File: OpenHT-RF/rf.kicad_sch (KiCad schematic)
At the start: 22 parts, among them J6 Conn_Coaxial, J7 Conn_01x02, J8 Conn_01x02, X1 ECS-TXO-20CSMV

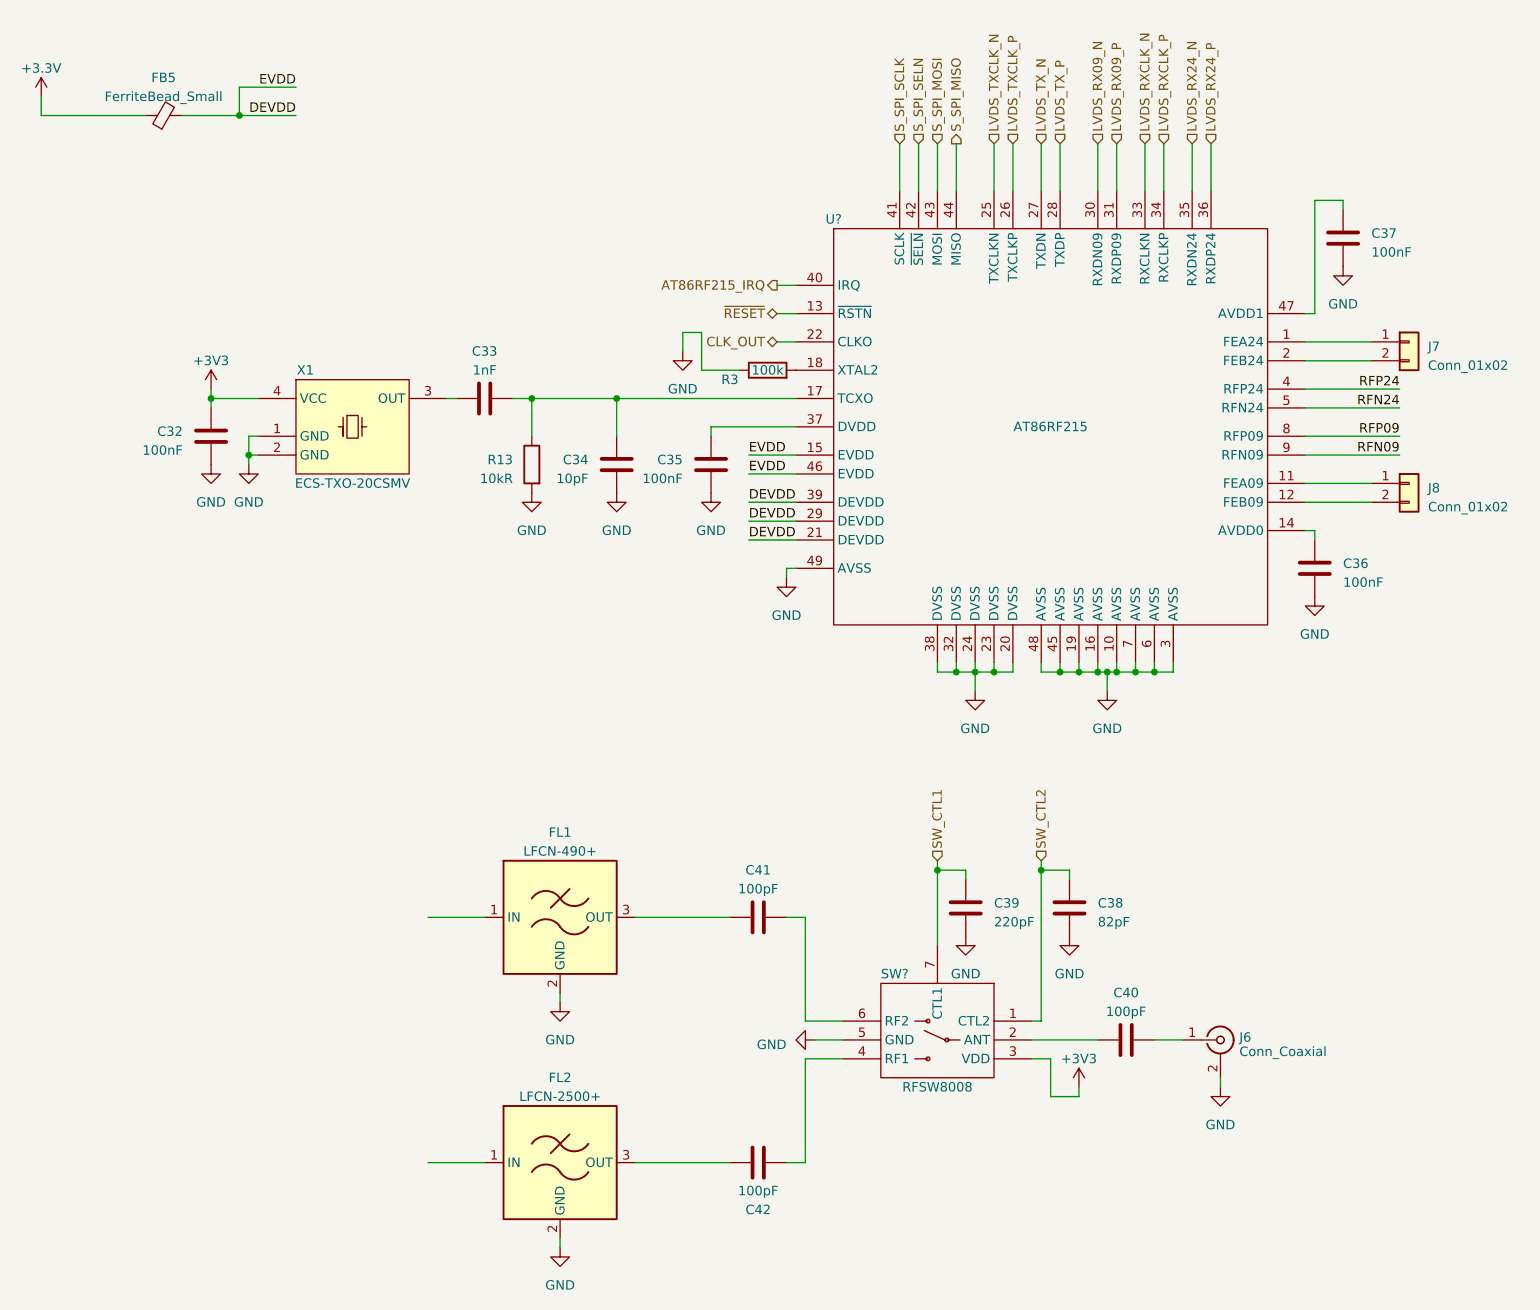
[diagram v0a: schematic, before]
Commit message: Added RF baluns
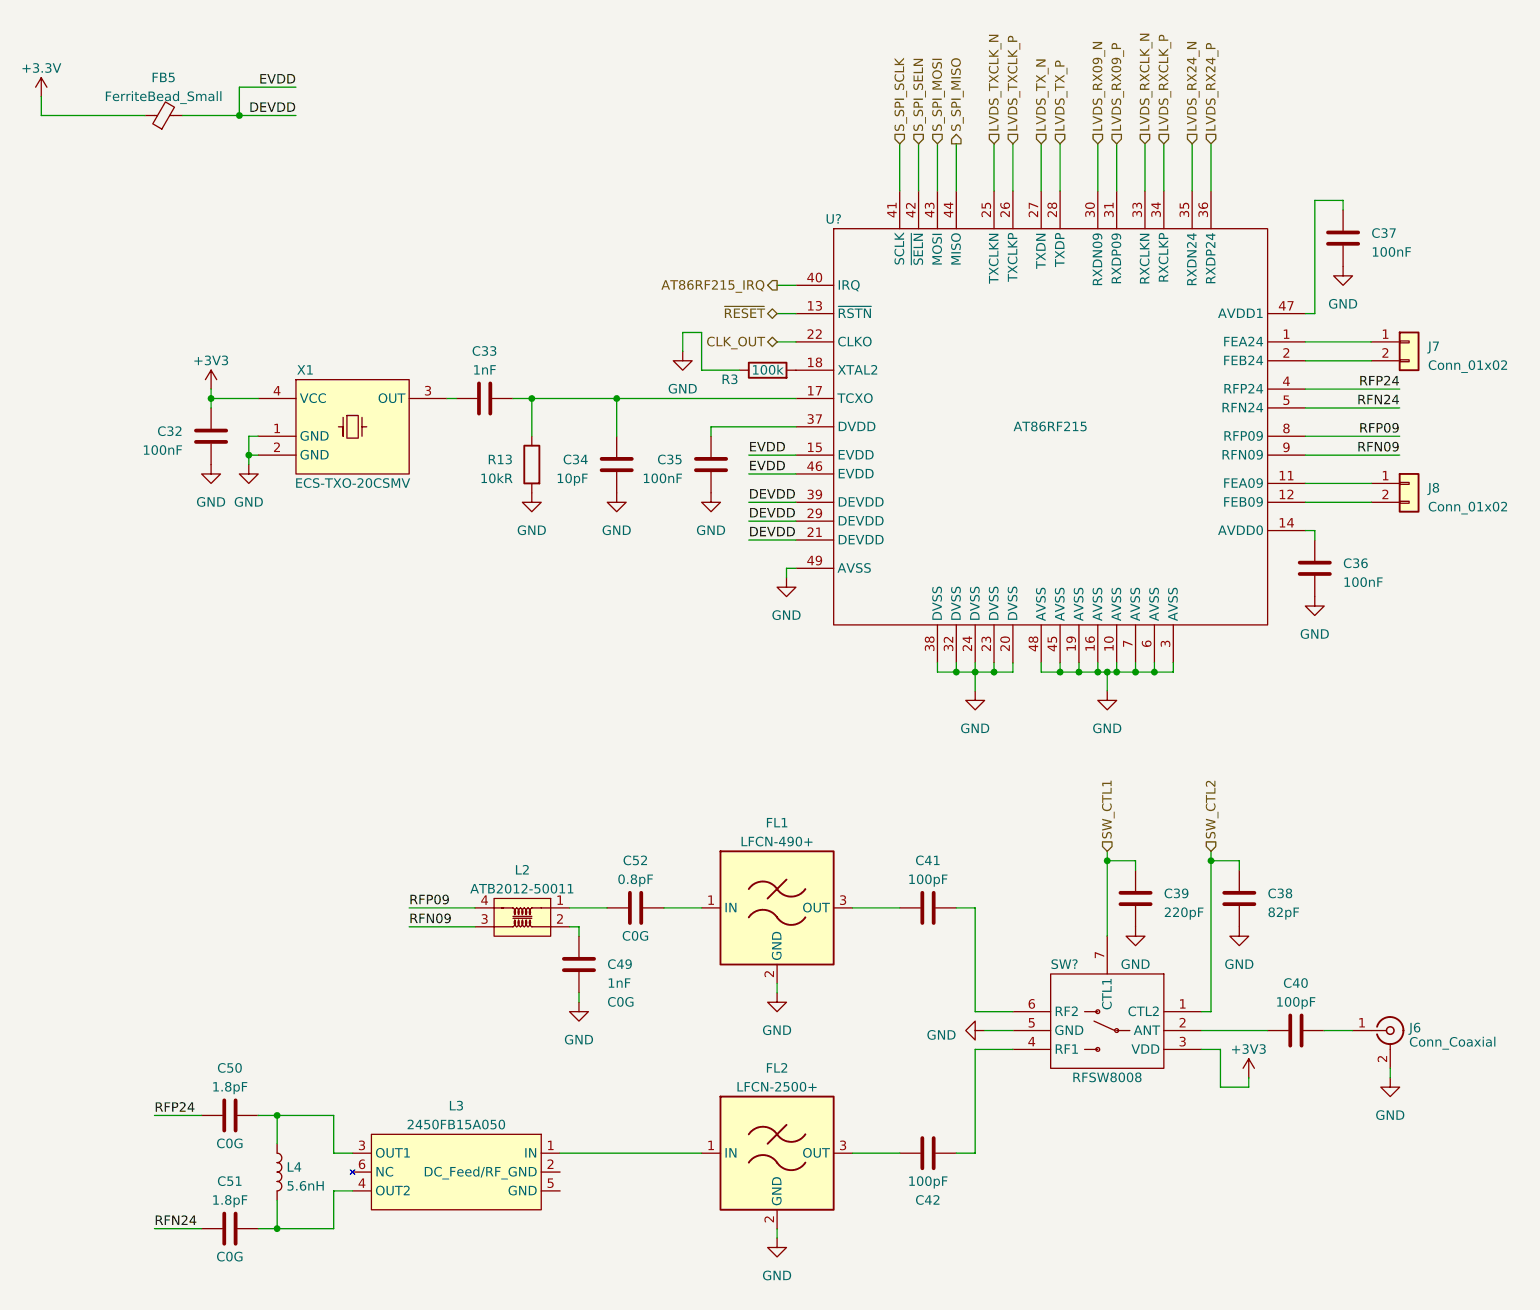
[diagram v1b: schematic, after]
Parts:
- added C49: 1nF, symbol Device:C
- added C50, C51: 1.8pF, symbol Device:C
- added C52: 0.8pF, symbol Device:C
- added L2: ATB2012-50011, M17_misc_passive:ATB2012, symbol M17_RF:ATB2012-50011
- added L3: 2450FB15A050, M17_misc_passive:2450FB15A050, symbol M17_RF:2450FB15A050
- added L4: 5.6nH, symbol Device:L
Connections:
- net GND: now also C49.2
- net RFN09: now also L2.3
- net RFN24: now also C51.1
- net RFP09: now also L2.4
- net RFP24: now also C50.1
- net at FL1.1 (IN): now also C52.2
- net at FL2.1 (IN): now also L3.1 (IN)
- new net: C51.2, L3.4 (OUT2), L4.2
- new net: C52.1, L2.1
- new net: C49.1, L2.2
- new net: C50.2, L3.3 (OUT1), L4.1
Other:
- moved on the sheet: C38, C39, C40, C41, C42, FL1, FL2, J6, SW?
